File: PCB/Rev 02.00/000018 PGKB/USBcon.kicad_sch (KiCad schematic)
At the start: 8 parts, among them J1 USB_B_V_Adam_USB-B-S-VT

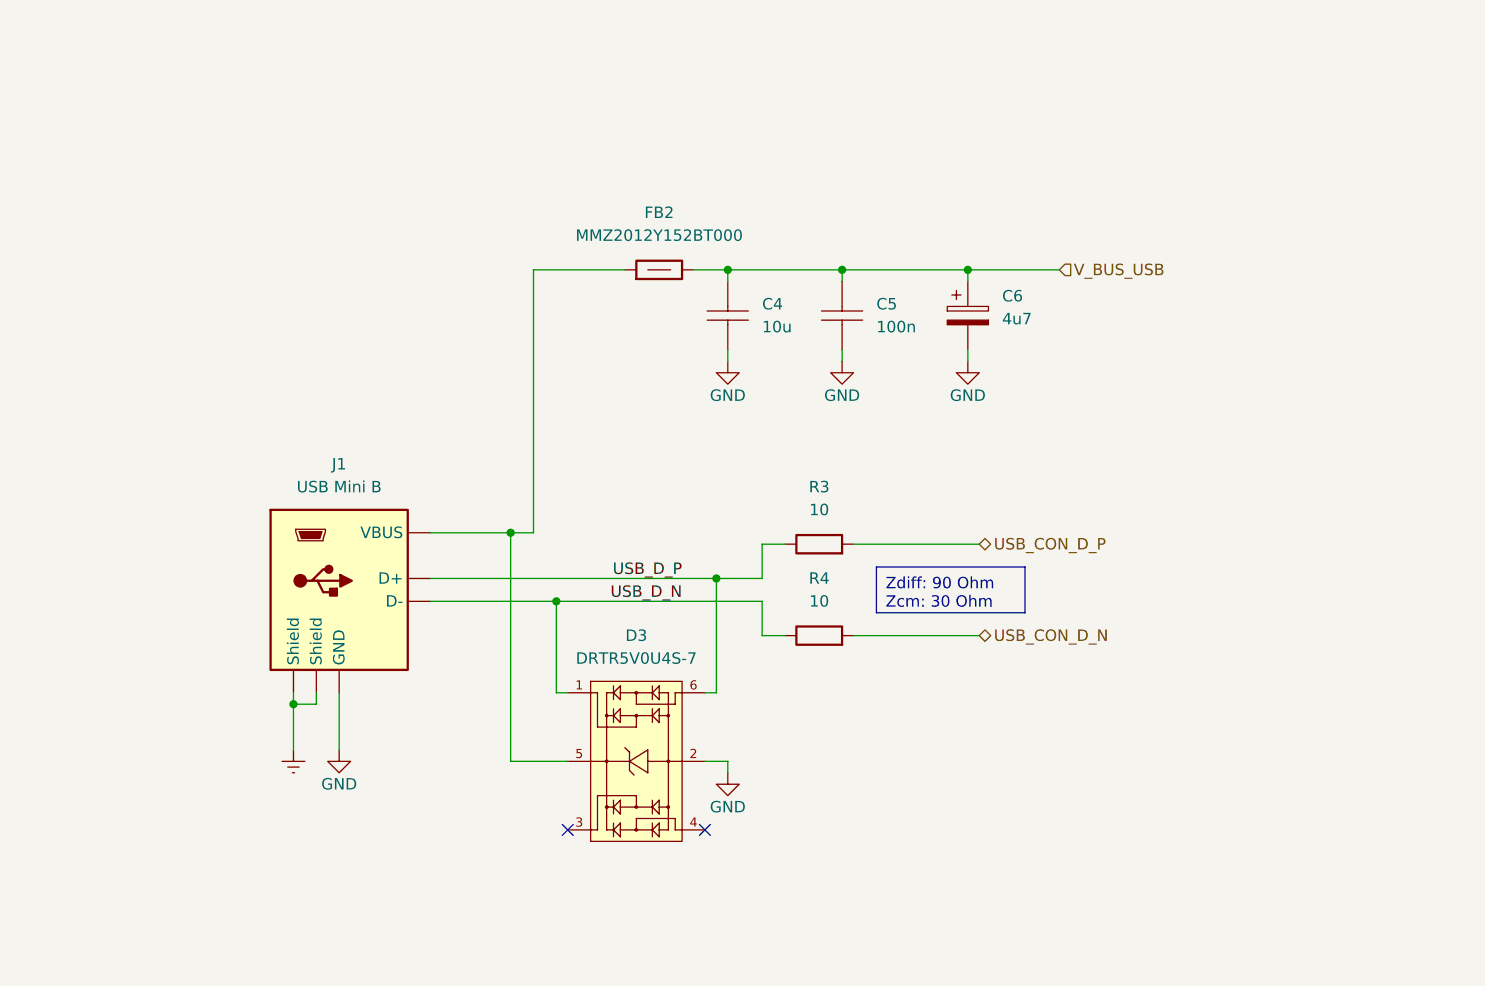
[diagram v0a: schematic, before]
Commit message: schematic
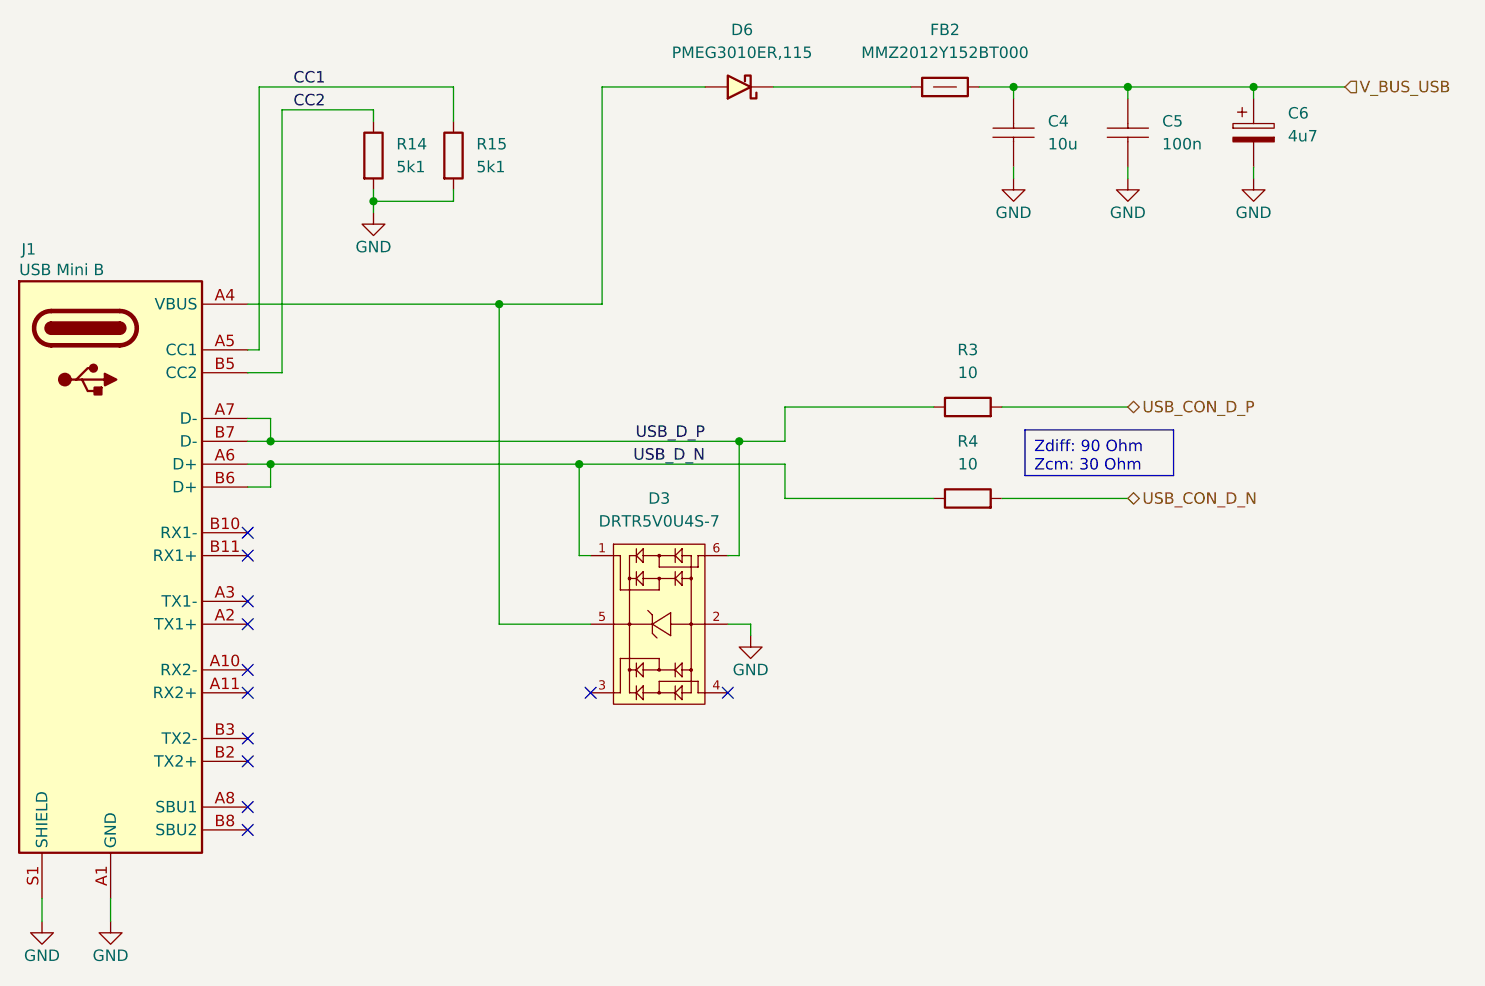
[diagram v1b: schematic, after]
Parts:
- removed J1: USB_B_V_Adam_USB-B-S-VT, KD_Connector_USB_HDMI_Etc:USB_B_Vertical_Adam_USB-B-S-VT, symbol KD_Connector_USB_HDMI_Etc:USB_B_V_Adam_USB-B-S-VT
- added D6: Schottky_30V_1A_PMEG3010ER_115, KD_Diode:DIOC360X180X150_SOD123, symbol KD_Diode:Schottky_30V_1A_PMEG3010ER_115
- added J1: USB Mini B, KD_Connector_USB_HDMI_Etc:USB_C_Receptacle_GCT_USB4085, symbol KD_Connector_USB_HDMI_Etc:USB_C_V_GCT_USB4085-GF-A
- added R14, R15: R_0603_5100_1%, KD_Resistor:RESC1608X55N, symbol KD_Resistor:R_0603_5100_1%
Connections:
- net GND: now also J1.A1 (GND), J1.A12 (GND), J1.B1 (GND), J1.B12 (GND), J1.S1 (SHIELD), R14.2, R15.2
- net USB_D_N: now also J1.A6 (D+), J1.B6 (D+)
- net USB_D_P: now also J1.A7 (D-), J1.B7 (D-)
- net at D3.5 (V+): now also D6.2 (A), J1.A4 (VBUS), J1.A9 (VBUS), J1.B4 (VBUS), J1.B9 (VBUS); no longer FB2.1
- new net: D6.1 (K), FB2.1
- new net CC1: J1.A5 (CC1), R15.1
- new net CC2: J1.B5 (CC2), R14.1
- no-connect marks 2 -> 12
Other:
- moved on the sheet: C4, C5, C6, D3, FB2, R3, R4
